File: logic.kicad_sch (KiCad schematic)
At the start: 68 parts, among them J5 HanRun_HR911105A, Q24 2N7002, Q25 AO3401A, SW2 SW_Push, U10 LAN8720A, U11 74HC595, U17 N066-6448TSWEG03-H28, U8 SY8120B1ABC, U9 ESP32-WROOM-32E

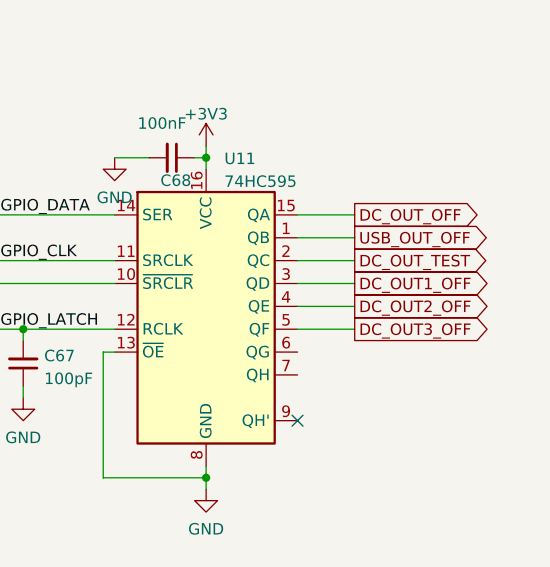
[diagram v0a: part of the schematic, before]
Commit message: Finish initial layout
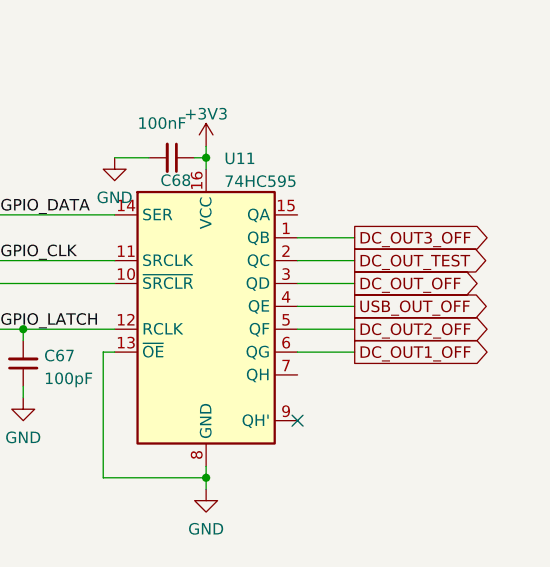
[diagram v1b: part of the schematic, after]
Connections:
- net DC_OUT1_OFF: now also U11.6 (QG); no longer U11.3 (QD)
- net DC_OUT2_OFF: now also U11.5 (QF); no longer U11.4 (QE)
- net DC_OUT3_OFF: now also U11.1 (QB); no longer U11.5 (QF)
- net DC_OUT_OFF: now also U11.3 (QD); no longer U11.15 (QA)
- net USB_OUT_OFF: now also U11.4 (QE); no longer U11.1 (QB)
